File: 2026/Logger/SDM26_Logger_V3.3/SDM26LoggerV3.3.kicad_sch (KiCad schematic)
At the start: 134 parts, among them IC1 ESP32-S3-WROOM-1-N8R8, IC2 CP2102N-A02-GQFN28, IC3 MIC37100-3.3WS, IC4 TPS563211DRLR, IC5 TLP175A_TPL,E, IC6 MIC37100-3.3WS, IC7 NEO-F9P-15B, IC8 TPS259250DRCR, J1 UART_USB, J2 ESP_USB, J3 GNSS_Debug, J4 Molex_1040310811, J5 1-776087-4, J6 1-776087-4, Q1 MMBT2222LT1G, Q2 MMBT2222LT1G, U1 INA260, U10 EMIF06-MSD02N16, U2 USBLC6-2SC6, U3 TPS2116DRL, U4 USBLC6-2SC6, U5 USBLC6-2SC6, U6 TPS2116, U7 SN65HVD230, U8 ADR425BRZ, U9 ADC128S102, Y1 ECX-.327-CDX-2096

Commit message: BSPD Formatting and misc
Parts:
- D1: symbol SDM_DIODES:ESDCAN03-2BWY -> SDM_ESD:ESDCAN03-2BWY

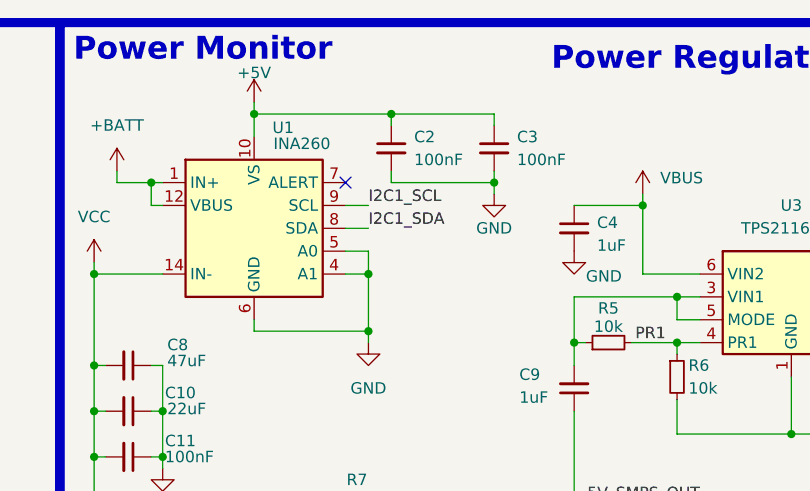
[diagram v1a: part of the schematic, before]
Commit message: NDTC BCP Start
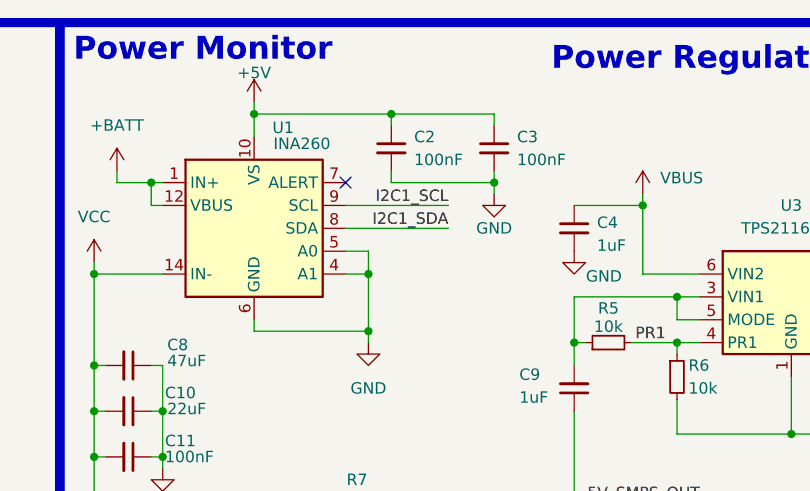
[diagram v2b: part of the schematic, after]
